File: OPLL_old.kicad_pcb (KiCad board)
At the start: 4 copper layers, 50 parts, among them J1 Conn_Coaxial, J2 Conn_Coaxial, J3 B4B-PH-K-S_LF__SN_, J4 Conn_Coaxial, J5 Conn_Coaxial, J6 Conn_Coaxial, J7 OSTTC042162, U1 ADF4107, U2 Opamp_Quad, U3 OPA847xDBV, U4 MC7805CD2TR4G D+, U5 MC7805CD2TR4G A+, U6 MC7905ACD2TR4G A-, U7 LP2950ACDT-3.3RG

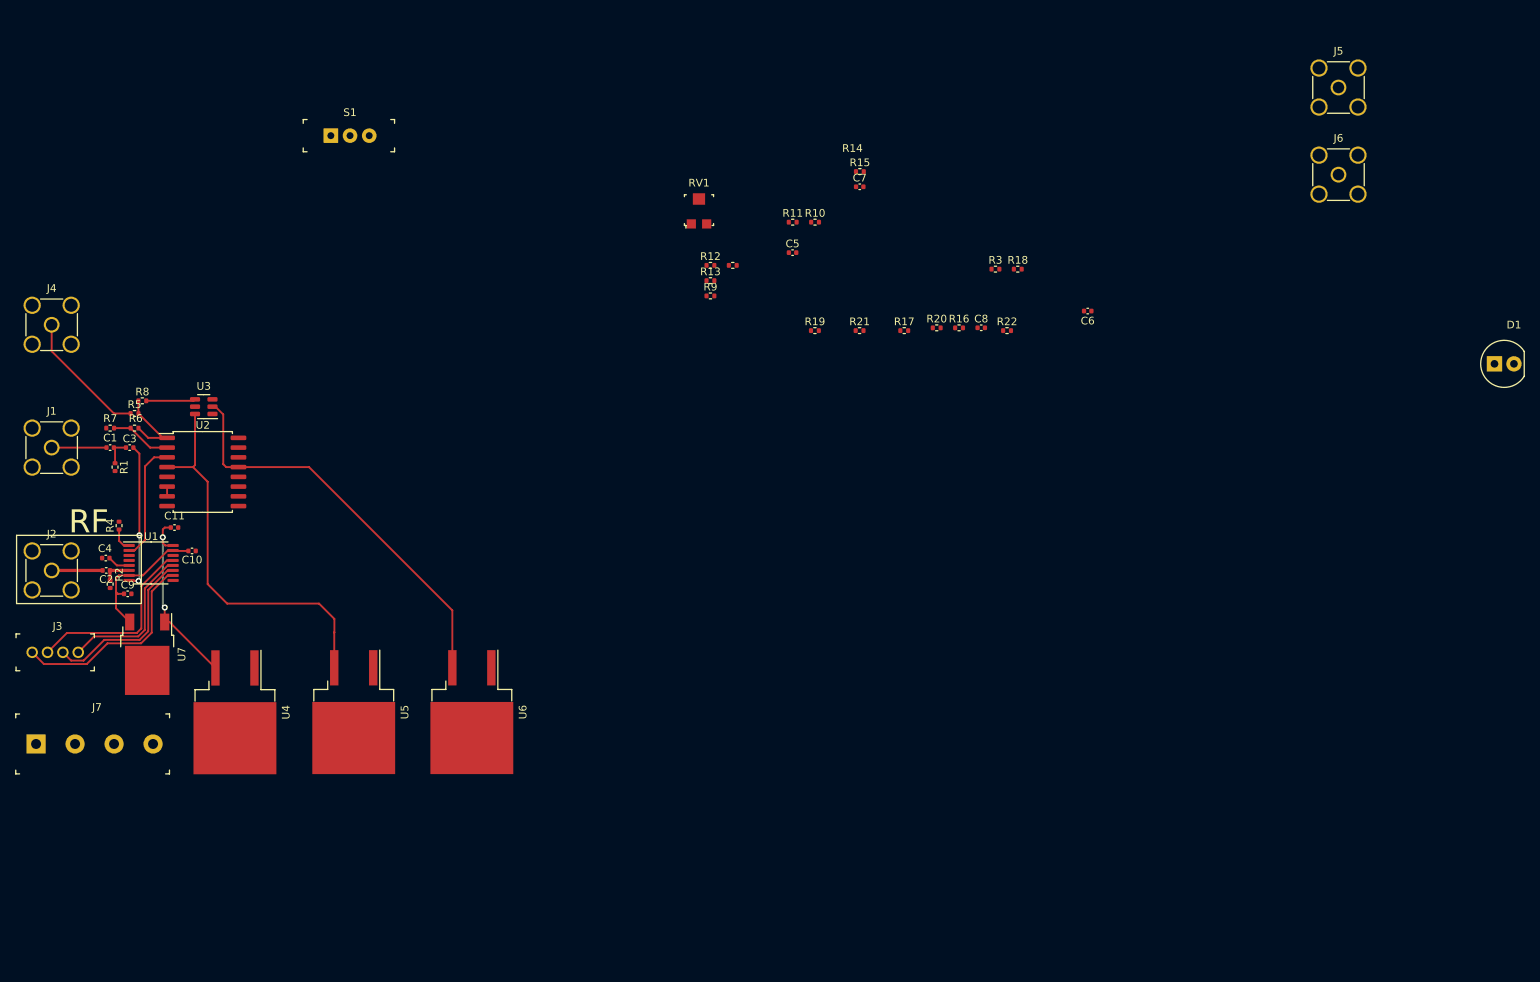
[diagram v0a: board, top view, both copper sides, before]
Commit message: First OPLL iteration
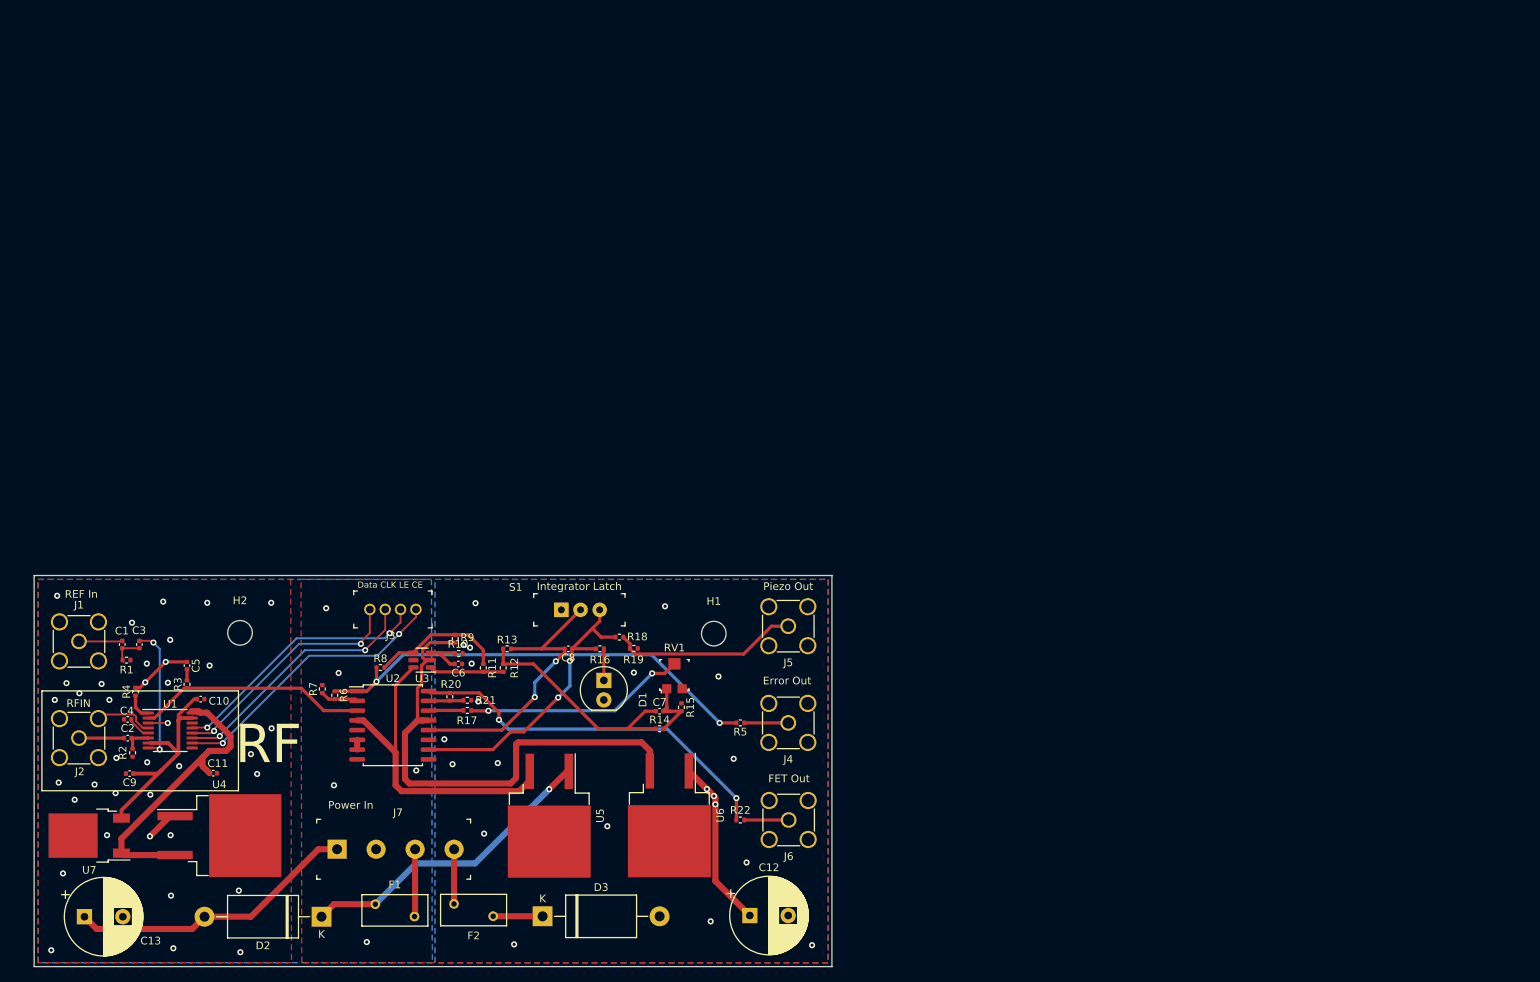
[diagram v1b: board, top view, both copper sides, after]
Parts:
- added C12: C_Polarized_Small_US, Capacitor_THT:CP_Radial_D10.0mm_P5.00mm, F.Cu at (136.7, 147.3)
- added C13: C_Polarized_Small_US, Capacitor_THT:CP_Radial_D10.0mm_P5.00mm, F.Cu at (50.0, 147.5)
- added D2: SA15CA-TP, Diode_THT:D_DO-201AE_P15.24mm_Horizontal, F.Cu at (80.9, 147.5)
- added D3: SA15CA-TP, Diode_THT:D_DO-201AE_P15.24mm_Horizontal, F.Cu at (109.7, 147.4)
- added F1: Polyfuse RXEF040, Fuse:Fuse_BelFuse_0ZRE0005FF_L8.3mm_W3.8mm, F.Cu at (87.9, 145.8)
- added F2: Polyfuse RXEF040, Fuse:Fuse_BelFuse_0ZRE0005FF_L8.3mm_W3.8mm, F.Cu at (103.2, 147.4)
- added H1: MountingHole, MountingHole:MountingHole_3.2mm_M3, F.Cu at (132.0, 110.6)
- added H2: MountingHole, MountingHole:MountingHole_3.2mm_M3, F.Cu at (70.3, 110.5)
- moved D1 126.4 mm to (117.7, 119.2), turned to -90 degrees
- moved R3 118.4 mm to (63.3, 117.2), turned to 90 degrees
- moved J6 110.4 mm to (141.7, 134.9), turned to 180 degrees
- moved J4 109.1 mm to (141.7, 122.2), turned to 180 degrees
- moved J5 100.3 mm to (141.7, 109.6), turned to 180 degrees
- moved C5 95.5 mm to (63.3, 114.8), turned to -90 degrees
- moved C6 94.0 mm to (98.7, 114.6), turned to 180 degrees
- moved R5 88.6 mm to (135.4, 122.2), turned to 180 degrees
- moved R20 79.6 mm to (97.6, 118.8), turned to -90 degrees
- moved R17 75.4 mm to (99.9, 120.6)
- moved R15 73.6 mm to (127.8, 120.2), turned to -90 degrees
- moved C7 73.1 mm to (124.9, 120.7)
- moved R10 72.9 mm to (98.8, 113.2), turned to 180 degrees
- moved R22 72.6 mm to (135.4, 134.9), turned to 180 degrees
- moved R11 70.7 mm to (102.0, 115.1), turned to -90 degrees
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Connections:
- J7 pad 3: +15V -> Net-(J7-Pad3)
- J7 pad 4: -15V -> Net-(J7-Pad4)
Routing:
- net Net-(R20-Pad1): track 0.00 -> 49.3 mm, vias 0 -> 2
- net Net-(R5-Pad2): track 11.0 -> 59.8 mm, vias 0 -> 2
- net GND2: track 0.00 -> 48.5 mm, vias 0 -> 26
- net +15V: track 0.00 -> 44.4 mm, vias 0 -> 2
- net Net-(C8-Pad1): track 0.00 -> 40.0 mm, vias 0 -> 2
- net Net-(C8-Pad2): track 0.00 -> 37.7 mm, vias 0 -> 2
- net Net-(C7-Pad1): track 0.00 -> 30.0 mm
- net Net-(R17-Pad2): track 0.00 -> 29.0 mm, vias 0 -> 2
- net -15V: track 0.00 -> 28.6 mm, vias 0 -> 3
- net Net-(J5-Pad1): track 0.00 -> 24.3 mm
- net Net-(R3-Pad1): track 15.6 -> 30.0 mm
- net +5VD: track 24.6 -> 38.4 mm, vias 2 -> 0
- net -5VA: track 53.5 -> 65.5 mm
- net Net-(J3-Pad4): track 20.2 -> 32.1 mm, vias 0 -> 2
- net Net-(J4-Pad1): track 17.1 -> 5.74 mm
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- added copper zone on B.Cu, net +15V
- added copper zone on B.Cu, net -15V
- added copper zone on F.Cu, net GND1
- added copper zone on In1.Cu, net GND1
- added copper zone on F.Cu, net GND2
- added copper zone on In2.Cu, net GND2
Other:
- board outline added: 103.9 x 51 mm
- board text added: "Data CLK LE CE"
- board text added: "Error Out"
- board text added: "FET Out"
- board text added: "Integrator Latch"
- board text added: "Piezo Out"
- board text added: "Power In"
- board text added: "REF In"
- board text added: "RFIN"

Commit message: it2
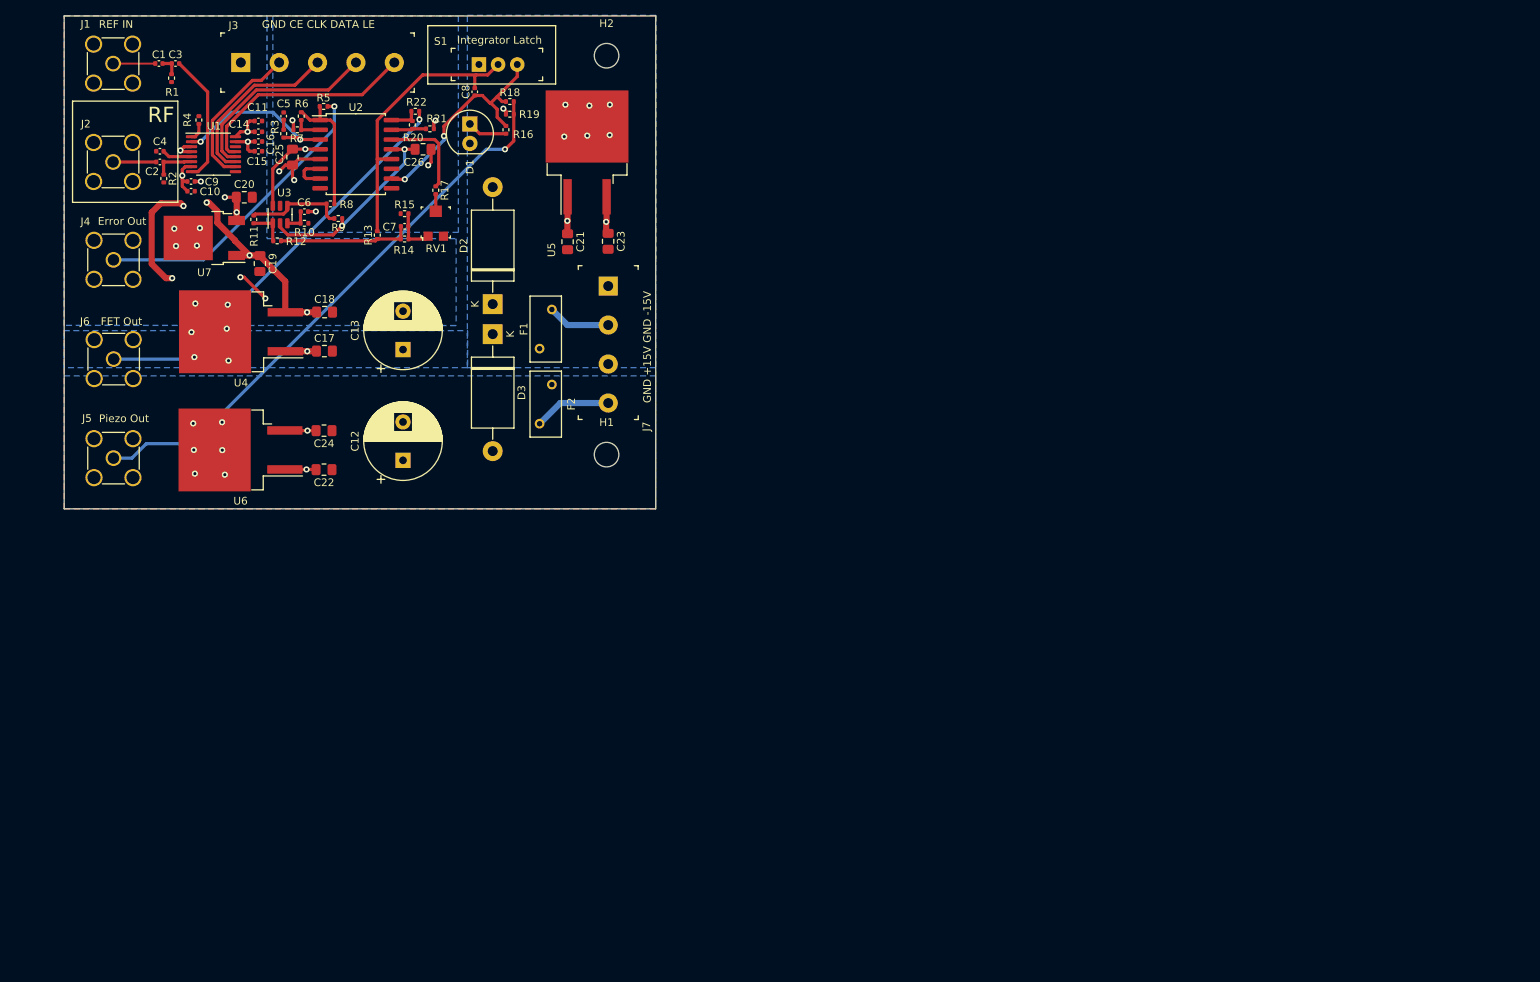
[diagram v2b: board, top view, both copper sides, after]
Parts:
- added C14: 10p, Capacitor_SMD:C_0402_1005Metric, F.Cu at (72.6, 45.2)
- added C15: 0.1u, Capacitor_SMD:C_0402_1005Metric, F.Cu at (72.6, 47.8)
- added C16: 10p, Capacitor_SMD:C_0402_1005Metric, F.Cu at (72.6, 46.5)
- added C17: T58W9105M035C0500, Capacitor_SMD:C_0805_2012Metric_Pad1.18x1.45mm_HandSolder, F.Cu at (81.3, 73.8)
- added C18: T58W9105M035C0500, Capacitor_SMD:C_0805_2012Metric_Pad1.18x1.45mm_HandSolder, F.Cu at (81.3, 68.7)
- added C19: T58W9105M035C0500, Capacitor_SMD:C_0805_2012Metric_Pad1.18x1.45mm_HandSolder, F.Cu at (72.8, 62.4)
- added C20: T58W9105M035C0500, Capacitor_SMD:C_0805_2012Metric_Pad1.18x1.45mm_HandSolder, F.Cu at (70.8, 53.7)
- added C21: T58W9105M035C0500, Capacitor_SMD:C_0805_2012Metric_Pad1.18x1.45mm_HandSolder, F.Cu at (112.9, 59.5)
- added C22: T58W9105M035C0500, Capacitor_SMD:C_0805_2012Metric_Pad1.18x1.45mm_HandSolder, F.Cu at (81.2, 89.2)
- added C23: T58W9105M035C0500, Capacitor_SMD:C_0805_2012Metric_Pad1.18x1.45mm_HandSolder, F.Cu at (118.2, 59.5)
- added C24: T58W9105M035C0500, Capacitor_SMD:C_0805_2012Metric_Pad1.18x1.45mm_HandSolder, F.Cu at (81.2, 84.2)
- added C25: T58W9105M035C0500, Capacitor_SMD:C_0805_2012Metric_Pad1.18x1.45mm_HandSolder, F.Cu at (77.1, 48.5)
- added C26: T58W9105M035C0500, Capacitor_SMD:C_0805_2012Metric_Pad1.18x1.45mm_HandSolder, F.Cu at (94.1, 47.5)
- C10, C11: value 100p -> 0.1u
- C9: value 100p -> 10p
- J3: value B4B-PH-K-S_LF__SN_ -> OSTTC050162; footprint digikey-footprints:PinHeader_1x4_P2mm_Drill1mm -> digikey-footprints:Term_Block_1x5_P5mm
- moved J4 106.6 mm to (53.8, 61.9), turned to 0 degrees
- moved J6 106.5 mm to (53.8, 74.8), turned to 0 degrees
- moved R22 101.6 mm to (93.1, 42.5)
- moved R5 96.9 mm to (81.2, 41.9)
- moved J5 90.6 mm to (53.8, 87.7), turned to 0 degrees
- moved H2 89.1 mm to (118.0, 35.3)
- moved U5 86.6 mm to (115.5, 47.9), turned to 90 degrees
- moved C11 85.2 mm to (72.6, 43.8), turned to 0 degrees
- moved C13 84.7 mm to (91.5, 73.6), turned to 90 degrees
- moved D2 82.9 mm to (103.2, 67.7), turned to 90 degrees
- moved J7 81.4 mm to (118.2, 65.3), turned to -90 degrees
- moved U7 79.3 mm to (65.6, 59.1)
- moved C9 77.6 mm to (63.9, 51.7), turned to 0 degrees
- moved D3 76.1 mm to (103.2, 71.6), turned to -90 degrees
- moved R1 76.0 mm to (61.3, 38.2), turned to -90 degrees
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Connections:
- C10 pad 1: GND1 -> +3V3
- C10 pad 2: +3V3 -> GND
- C11 pad 1: GND1 -> +5VD
- C11 pad 2: +5VD -> GND
- C12 pad 1: -15V -> GND
- C12 pad 2: GND2 -> -15V
- C13 pad 1: GND2 -> +15V
- C13 pad 2: +15V -> GND
- C4 pad 2: GND1 -> GND
- C5 pad 1: GND2 -> GND
- C6 pad 1: GND2 -> GND
- C9 pad 2: GND1 -> GND
- D1 pad 2: GND2 -> GND
- D2 pad 2: GND2 -> GND
- D3 pad 1: -15V -> GND
- D3 pad 2: GND2 -> -15V
- F1 pad 2: Net-(J7-Pad3) -> Net-(F1-Pad2)
- J1 pad 2: GND1 -> GND
- J2 pad 2: GND1 -> GND
- J3 pad 1: Net-(J3-Pad1) -> GND
- J3 pad 2: Net-(J3-Pad2) -> Net-(U1-Pad10)
- J4 pad 2: GND2 -> GND
- J5 pad 2: GND2 -> GND
- J6 pad 2: GND2 -> GND
- J7 pad 1: GND2 -> GND
- J7 pad 2: GND1 -> Net-(F1-Pad2)
- J7 pad 3: Net-(J7-Pad3) -> GND
- R1 pad 2: GND1 -> GND
- R10 pad 1: GND2 -> GND
- R15 pad 1: GND2 -> GND
- R19 pad 2: GND2 -> GND
- R2 pad 2: GND1 -> GND
- R21 pad 2: GND2 -> GND
- R4 pad 2: GND2 -> GND
- R7 pad 2: GND2 -> GND
- RV1 pad 3: GND2 -> GND
- U1 pad 10: Net-(J3-Pad1) -> Net-(U1-Pad10)
- U1 pad 13: Net-(J3-Pad2) -> Net-(U1-Pad13)
- U1 pad 3: GND2 -> GND
- U1 pad 4: GND1 -> GND
- U1 pad 9: GND1 -> GND
- U2 pad 11: GND2 -> GND
- U2 pad 5: GND2 -> GND
- U4 pad 2: GND1 -> GND
- U5 pad 2: GND2 -> GND
- U6 pad 2: GND2 -> GND
- U7 pad 2: GND1 -> GND
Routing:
- net Net-(J5-Pad1): track 24.3 -> 74.4 mm, vias 0 -> 1
- net GND2: track 48.5 -> 0.00 mm, vias 26 -> 0
- net Net-(J6-Pad1): track 5.79 -> 54.1 mm, vias 0 -> 1
- net Net-(R20-Pad1): track 49.3 -> 4.09 mm, vias 2 -> 0
- net Net-(R5-Pad2): track 59.8 -> 17.2 mm, vias 2 -> 0
- net Net-(J3-Pad1): track 37.1 -> 0.00 mm, vias 2 -> 0
- net +15V: track 44.4 -> 8.91 mm
- net -5VA: track 65.5 -> 30.9 mm, vias 0 -> 3
- net Net-(J3-Pad2): track 34.5 -> 0.00 mm, vias 2 -> 0
- net Net-(J4-Pad1): track 5.74 -> 39.7 mm, vias 0 -> 1
- net GND: track 0.00 -> 30.2 mm, vias 0 -> 31
- net Net-(U1-Pad13): track 0.00 -> 29.5 mm
- net Net-(R17-Pad2): track 29.0 -> 2.23 mm, vias 2 -> 0
- net +5VA: track 42.6 -> 17.0 mm, vias 0 -> 2
- net -15V: track 28.6 -> 4.07 mm, vias 3 -> 1
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- added copper zone on In2.Cu, net +3V3
- added copper zone on In2.Cu, net +5VA
- added copper zone on B.Cu, net +5VD
- added copper zone on B.Cu, net -5VA
- added copper zone on In2.Cu, net -5VA
- added copper zone on F.Cu, net GND
- added copper zone on In1.Cu, net GND
- added copper zone on In2.Cu, net GND
- removed copper zone on F.Cu, net GND1
- removed copper zone on In1.Cu, net GND1
- removed copper zone on F.Cu, net GND2
- removed copper zone on In2.Cu, net GND2
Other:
- board size 103.9 x 51 mm -> 77.1 x 64.2 mm
- board text added: "GND +15V GND -15V"
- board text added: "GND CE CLK DATA LE"
- board text added: "REF IN"
- board text removed: "Data CLK LE CE"
- board text removed: "Power In"
- board text removed: "REF In"
- board text removed: "RFIN"
